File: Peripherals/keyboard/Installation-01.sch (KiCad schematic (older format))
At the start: 450 parts, among them J2 Conn_ARM_JTAG_SWD_10, U1 STM32F072CBTx, U2 MCP1700-3302E_SOT23, U3 MCP1700-1202E_SOT23, U4 TUSB4041I, U5 MCP1700-3302E_SOT23, U6 USBLC6-2SC6, Y1 24MHz

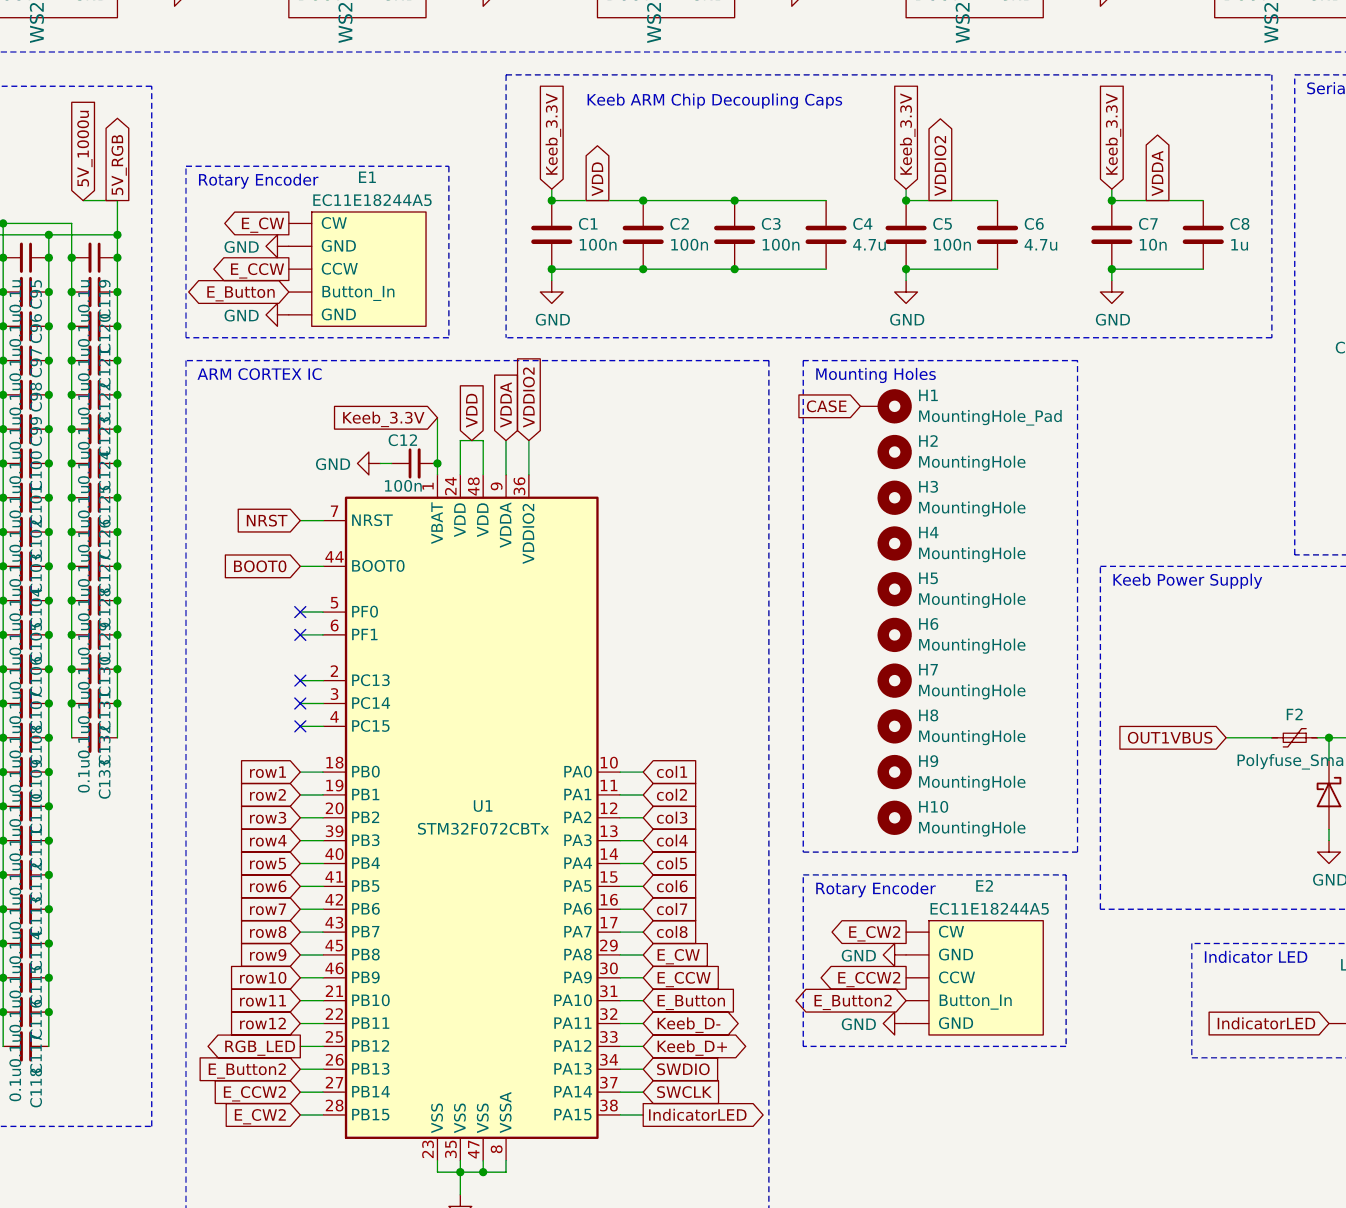
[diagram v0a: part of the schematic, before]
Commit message: encoder
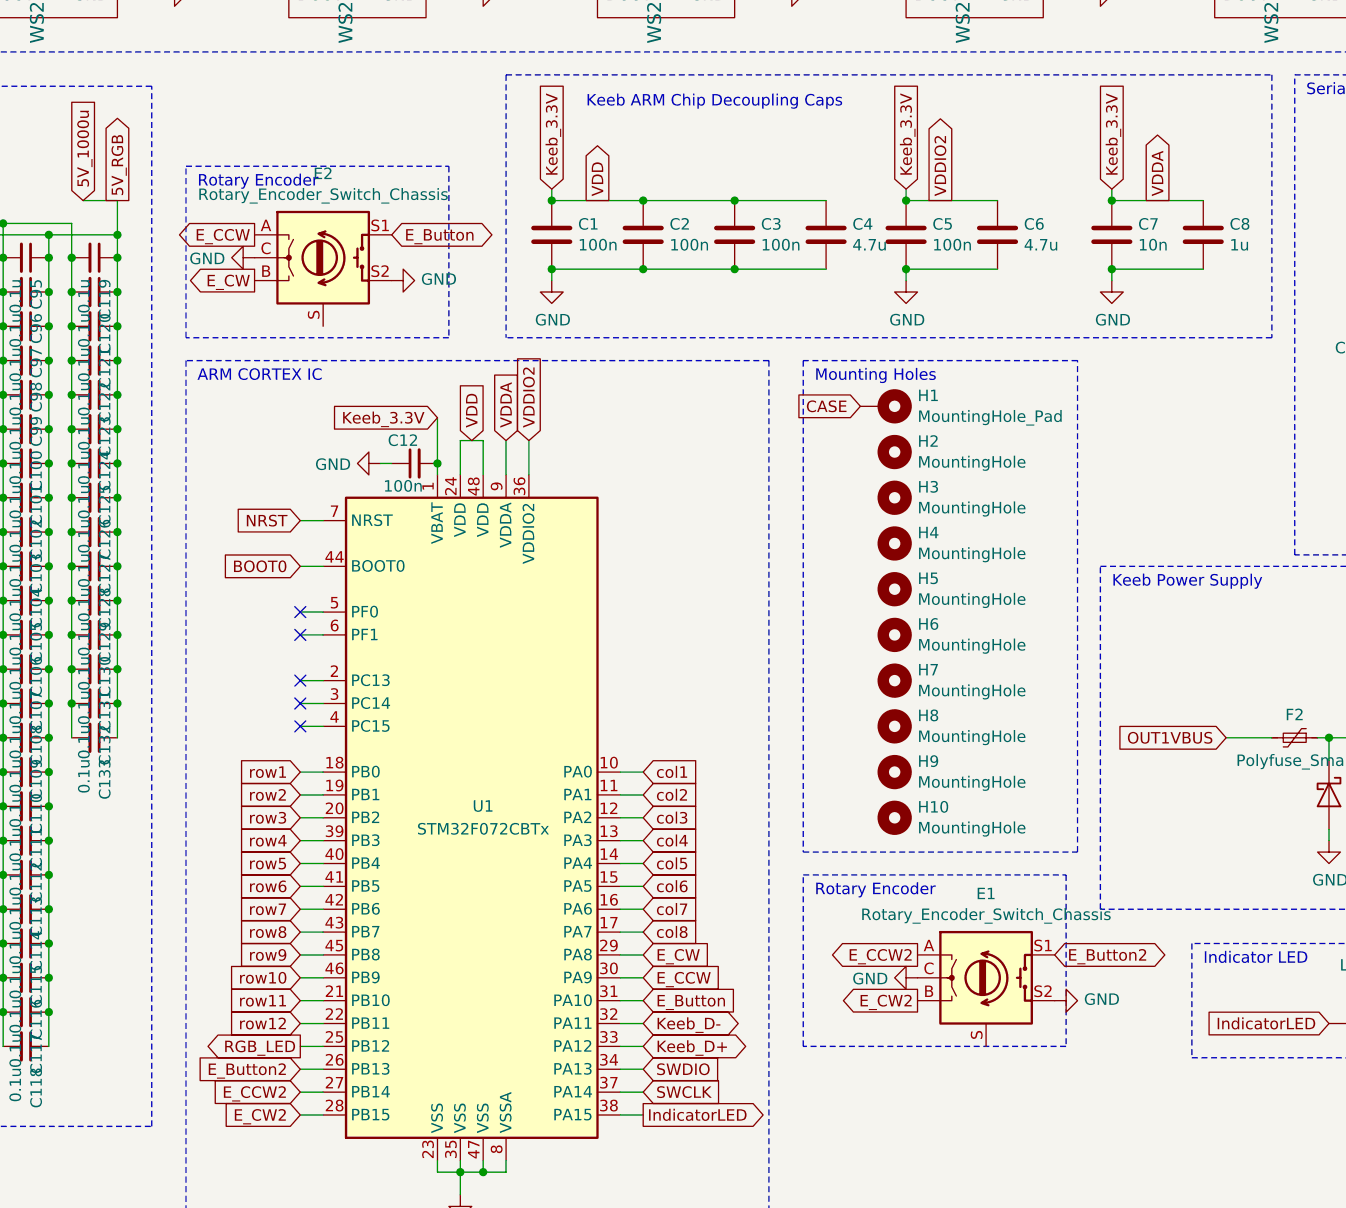
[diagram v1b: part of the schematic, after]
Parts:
- removed E1, E2: EC11E18244A5, symbol more-keeb-parts:EC11E18244A5-Incremental-Rotary-Encoder
- added E1, E2: Rotary_Encoder_Switch_Chassis, acheron_Hardware:ALPS_EC11E, symbol acheronSymbols:Rotary_Encoder_Switch_Chassis
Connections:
- net E_Button: now also E2.S1
- net E_Button2: now also E1.S1
- net E_CCW: now also E2.A
- net E_CCW2: now also E1.A
- net E_CW: now also E2.B
- net E_CW2: now also E1.B
- net GND: now also E1.C, E1.S2, E2.C, E2.S2
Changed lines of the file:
@@
 $EndComp
 $Comp
-L more-keeb-parts:EC11E18244A5-Incremental-Rotary-Encoder E1
-U 1 1 65147EF9
-P 17950 7250
-F 0 "E1" H 17900 7650 50  0000 L CNN
-F 1 "EC11E18244A5" H 17700 7550 50  0000 L CNN
-F 2 "" H 17600 7550 50  0001 C CNN
-F 3 "" H 17600 7550 50  0001 C CNN
-	1    17950 7250
-	1    0    0    -1
-$EndComp
-$Comp
 L power:GND #PWR0199
 U 1 1 6529FB78
-P 17600 7450
-F 0 "#PWR0199" H 17600 7200 50  0001 C CNN
-F 1 "GND" V 17605 7322 50  0000 R CNN
-F 2 "" H 17600 7450 50  0001 C CNN
-F 3 "" H 17600 7450 50  0001 C CNN
-	1    17600 7450
-	0    1    1    0
+P 18050 7300
+F 0 "#PWR0199" H 18050 7050 50  0001 C CNN
+F 1 "GND" V 18055 7172 50  0000 R CNN
+F 2 "" H 18050 7300 50  0001 C CNN
+F 3 "" H 18050 7300 50  0001 C CNN
+	1    18050 7300
+	0    -1   -1   0
 $EndComp
 $Comp
 L power:GND #PWR0200
 U 1 1 654C65A9
-P 17600 7150
-F 0 "#PWR0200" H 17600 6900 50  0001 C CNN
-F 1 "GND" V 17605 7022 50  0000 R CNN
-F 2 "" H 17600 7150 50  0001 C CNN
-F 3 "" H 17600 7150 50  0001 C CNN
-	1    17600 7150
+P 17450 7200
+F 0 "#PWR0200" H 17450 6950 50  0001 C CNN
+F 1 "GND" V 17455 7072 50  0000 R CNN
+F 2 "" H 17450 7200 50  0001 C CNN
+F 3 "" H 17450 7200 50  0001 C CNN
+	1    17450 7200
 	0    1    1    0
 $EndComp
@@
 Text GLabel 23500 6850 1    50   Input ~ 0
 Keeb_3.3V
-Text GLabel 17600 7050 0    50   Output ~ 0
+Text GLabel 17450 7300 0    50   Output ~ 0
 E_CW
 Text GLabel 19150 10250 2    50   Input ~ 0
 E_CW
-Text GLabel 17600 7250 0    50   Output ~ 0
+Text GLabel 17450 7100 0    50   Output ~ 0
 E_CCW
-Text GLabel 17600 7350 0    50   BiDi ~ 0
+Text GLabel 18050 7100 2    50   BiDi ~ 0
 E_Button
 Text GLabel 19150 10450 2    50   Input ~ 0
@@
 NoConn ~ 4900 2650
 $Comp
-L more-keeb-parts:EC11E18244A5-Incremental-Rotary-Encoder E2
-U 1 1 5EB31AAD
-P 20650 10350
-F 0 "E2" H 20600 10750 50  0000 L CNN
-F 1 "EC11E18244A5" H 20400 10650 50  0000 L CNN
-F 2 "" H 20300 10650 50  0001 C CNN
-F 3 "" H 20300 10650 50  0001 C CNN
-	1    20650 10350
-	1    0    0    -1
-$EndComp
-$Comp
 L power:GND #PWR0227
 U 1 1 5EB31AB3
-P 20300 10550
-F 0 "#PWR0227" H 20300 10300 50  0001 C CNN
-F 1 "GND" V 20305 10422 50  0000 R CNN
-F 2 "" H 20300 10550 50  0001 C CNN
-F 3 "" H 20300 10550 50  0001 C CNN
-	1    20300 10550
-	0    1    1    0
+P 20950 10450
+F 0 "#PWR0227" H 20950 10200 50  0001 C CNN
+F 1 "GND" V 20955 10322 50  0000 R CNN
+F 2 "" H 20950 10450 50  0001 C CNN
+F 3 "" H 20950 10450 50  0001 C CNN
+	1    20950 10450
+	0    -1   -1   0
 $EndComp
 $Comp
 L power:GND #PWR0228
 U 1 1 5EB31AB9
-P 20300 10250
-F 0 "#PWR0228" H 20300 10000 50  0001 C CNN
-F 1 "GND" V 20305 10122 50  0000 R CNN
-F 2 "" H 20300 10250 50  0001 C CNN
-F 3 "" H 20300 10250 50  0001 C CNN
-	1    20300 10250
+P 20350 10350
+F 0 "#PWR0228" H 20350 10100 50  0001 C CNN
+F 1 "GND" V 20355 10222 50  0000 R CNN
+F 2 "" H 20350 10350 50  0001 C CNN
+F 3 "" H 20350 10350 50  0001 C CNN
+	1    20350 10350
 	0    1    1    0
 $EndComp
-Text GLabel 20300 10150 0    50   Output ~ 0
+Text GLabel 20350 10450 0    50   Output ~ 0
 E_CW2
-Text GLabel 20300 10350 0    50   Output ~ 0
+Text GLabel 20350 10250 0    50   Output ~ 0
 E_CCW2
-Text GLabel 20300 10450 0    50   BiDi ~ 0
+Text GLabel 20950 10250 2    50   BiDi ~ 0
 E_Button2
 Text Notes 19900 10000 0    50   ~ 0
@@
 Text Notes 21600 10300 0    50   ~ 0
 Indicator LED
+$Comp
+L acheronSymbols:Rotary_Encoder_Switch_Chassis E1
+U 1 1 5ECC7078
+P 20650 10350
+F 0 "E1" H 20650 10717 50  0000 C CNN
+F 1 "Rotary_Encoder_Switch_Chassis" H 20650 10626 50  0000 C CNN
+F 2 "acheron_Hardware:ALPS_EC11E" H 20500 10510 50  0001 C CNN
+F 3 "~" H 20650 10610 50  0001 C CNN
+	1    20650 10350
+	1    0    0    -1
+$EndComp
+$Comp
+L acheronSymbols:Rotary_Encoder_Switch_Chassis E2
+U 1 1 5F873A39
+P 17750 7200
+F 0 "E2" H 17750 7567 50  0000 C CNN
+F 1 "Rotary_Encoder_Switch_Chassis" H 17750 7476 50  0000 C CNN
+F 2 "acheron_Hardware:ALPS_EC11E" H 17600 7360 50  0001 C CNN
+F 3 "~" H 17750 7460 50  0001 C CNN
+	1    17750 7200
+	1    0    0    -1
+$EndComp
 $EndSCHEMATC
